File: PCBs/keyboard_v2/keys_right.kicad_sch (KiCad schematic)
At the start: 55 parts, among them SW701 RIC11-31S15.5D7-TH, SW702 SW_DIP_x01, SW703 SW_DIP_x01, SW704 SW_DIP_x01, SW705 SW_DIP_x01, SW706 SW_DIP_x01, SW707 SW_DIP_x01, SW708 SW_DIP_x01, SW709 SW_DIP_x01, SW710 SW_DIP_x01, SW711 SW_DIP_x01, SW712 SW_DIP_x01, SW713 SW_DIP_x01, SW714 SW_DIP_x01, SW715 SW_DIP_x01, SW716 SW_DIP_x01, SW717 SW_DIP_x01, SW718 SW_DIP_x01, SW719 SW_DIP_x01, SW720 SW_DIP_x01, SW721 SW_DIP_x01, SW722 SW_DIP_x01, SW723 SW_DIP_x01, SW724 SW_DIP_x01, SW725 SW_DIP_x01, SW726 SW_DIP_x01, SW727 SW_DIP_x01, SW728 SW_DIP_x01

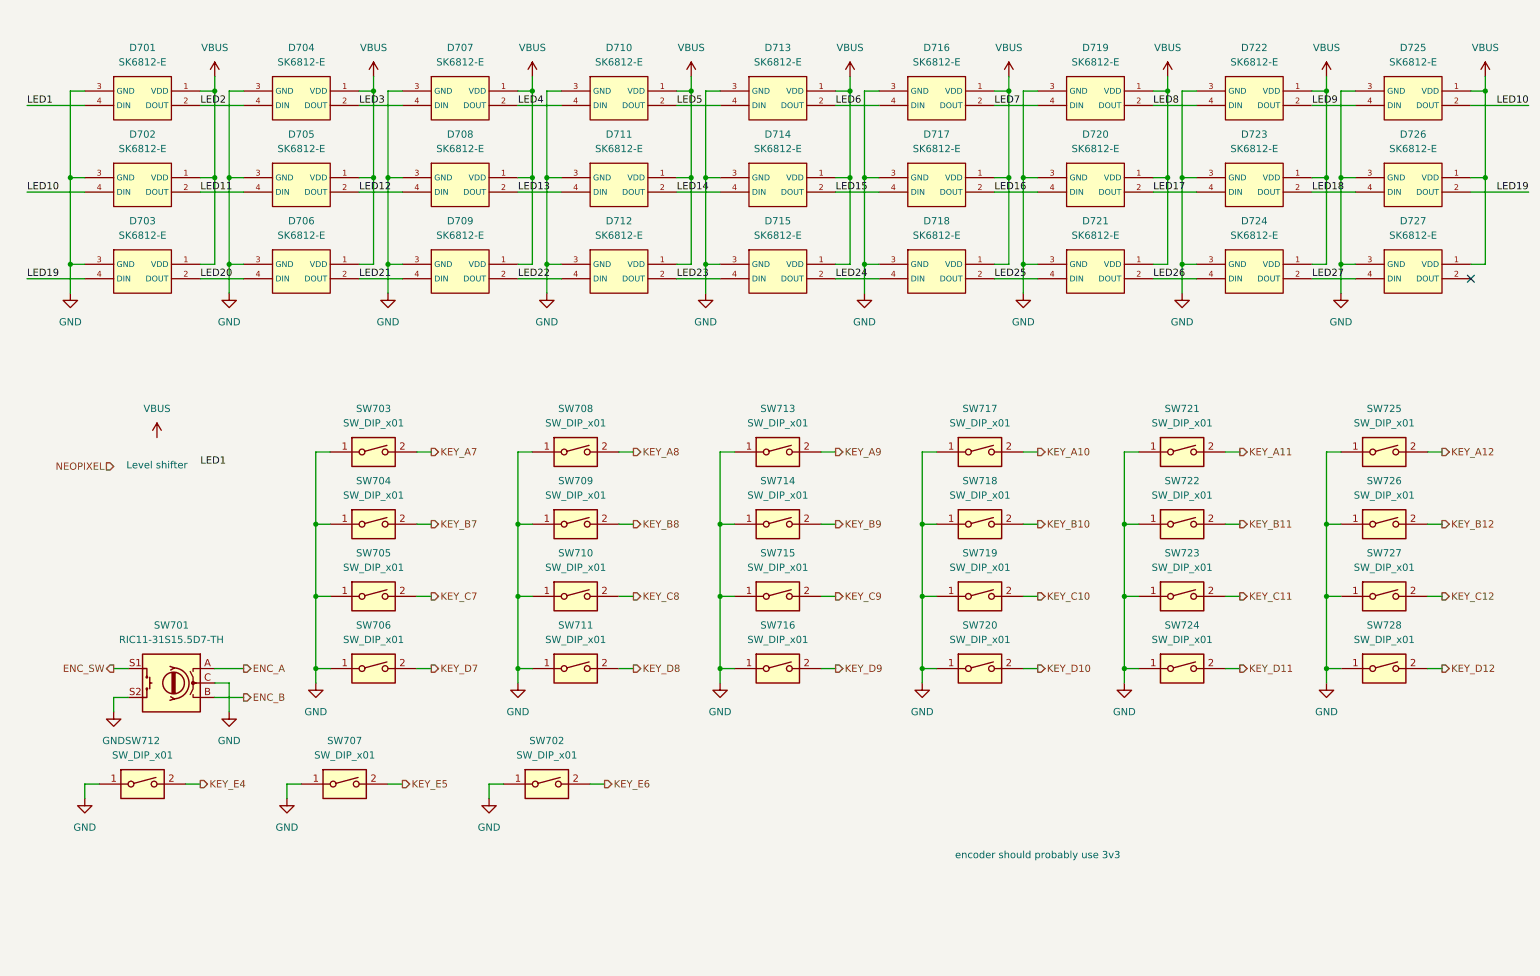
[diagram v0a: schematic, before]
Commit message: V2 Schematic mostly done
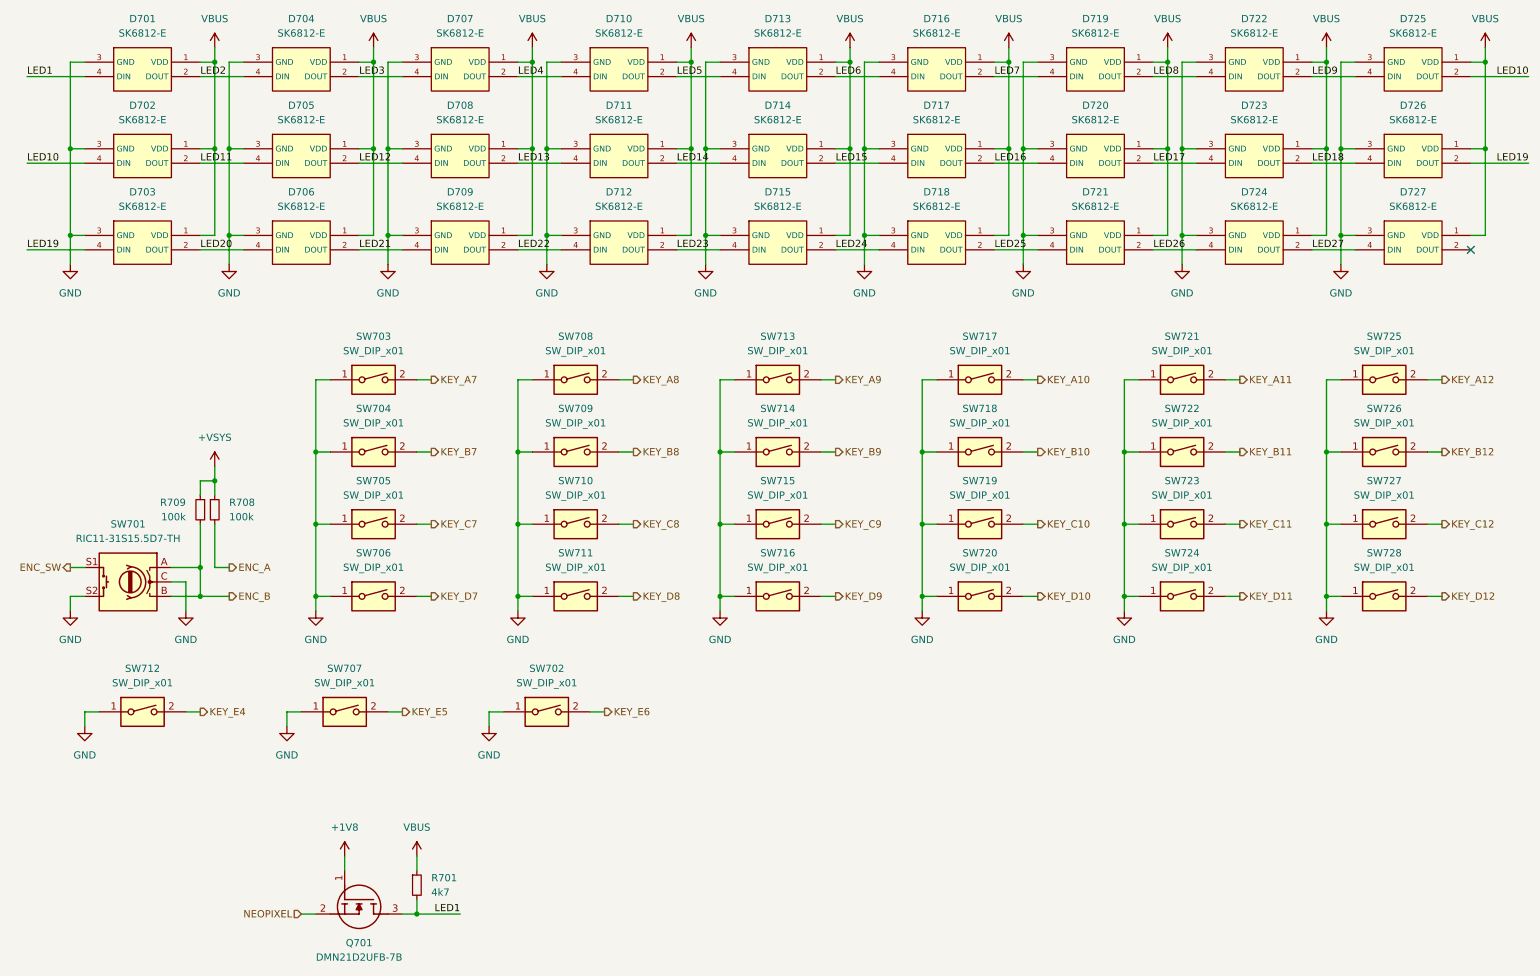
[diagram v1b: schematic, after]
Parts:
- added Q701: DMN21D2UFB-7B, keyboard_footprints:DMN21D2UFB7B, symbol DMN21D2UFB-7B:DMN21D2UFB-7B
- added R701: 4k7, Resistor_SMD:R_0402_1005Metric, symbol Device:R_Small
- added R708, R709: 100k, Resistor_SMD:R_0402_1005Metric, symbol Device:R_Small
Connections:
- net ENC_A: now also R708.2; no longer SW701.A
- net ENC_B: now also SW701.A, R709.2
- net LED1: now also Q701.3 (D), R701.2
- net NEOPIXEL: now also Q701.2 (S)
- net VBUS: now also R701.1
- new net +1V8: Q701.1 (G)
- new net +VSYS: R708.1, R709.1
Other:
- note removed: "Level shifter"
- note removed: "encoder should probably use 3v3"
- moved on the sheet: D701, D702, D703, D704, D705, D706, D707, D708, D709, D710, D711, D712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
